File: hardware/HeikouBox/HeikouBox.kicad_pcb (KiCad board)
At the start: 2 copper layers, 100 x 100 mm, 193 parts, among them J101 5V, J201 Conn_02x05_Odd_Even, J202 Conn_02x08_Odd_Even, J301 DB15_Female_HighDensity_Mount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, J302 AudioJack3_SwitchTR, J501 Micro_SD_Card_TFP09-2-12B, J503 PS/2, Q301 MMBT3904, Q302 MMBT3904, Q303 MMBT3904, Q304 MMBT3904, Q305 MMBT3904, Q306 MMBT3904, Q307 MMBT3904, Q502 BSS138, Q503 BSS138, SW501 Left, SW502 Right, SW503 Up, SW504 Down, U101 LD1117S33TR, U102 LD1117S25TR, U103 LD1117S12TR, U201 HeikouBox-Core, U202 74HCU04, U401 K4S281632-UC60, U501 STM32-BluePill-Socket, Y201 14.31818MHz, Y202 28.37516MHz

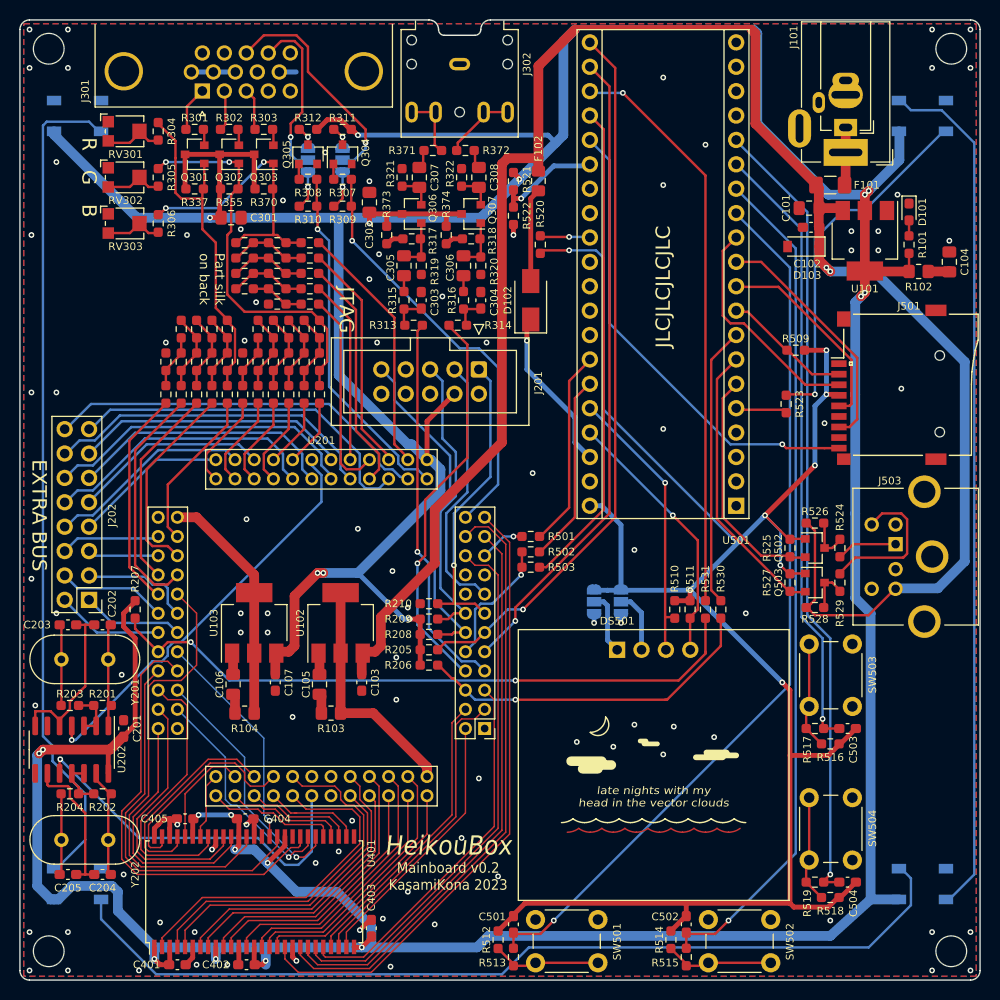
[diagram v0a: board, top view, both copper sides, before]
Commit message: Upload latest files
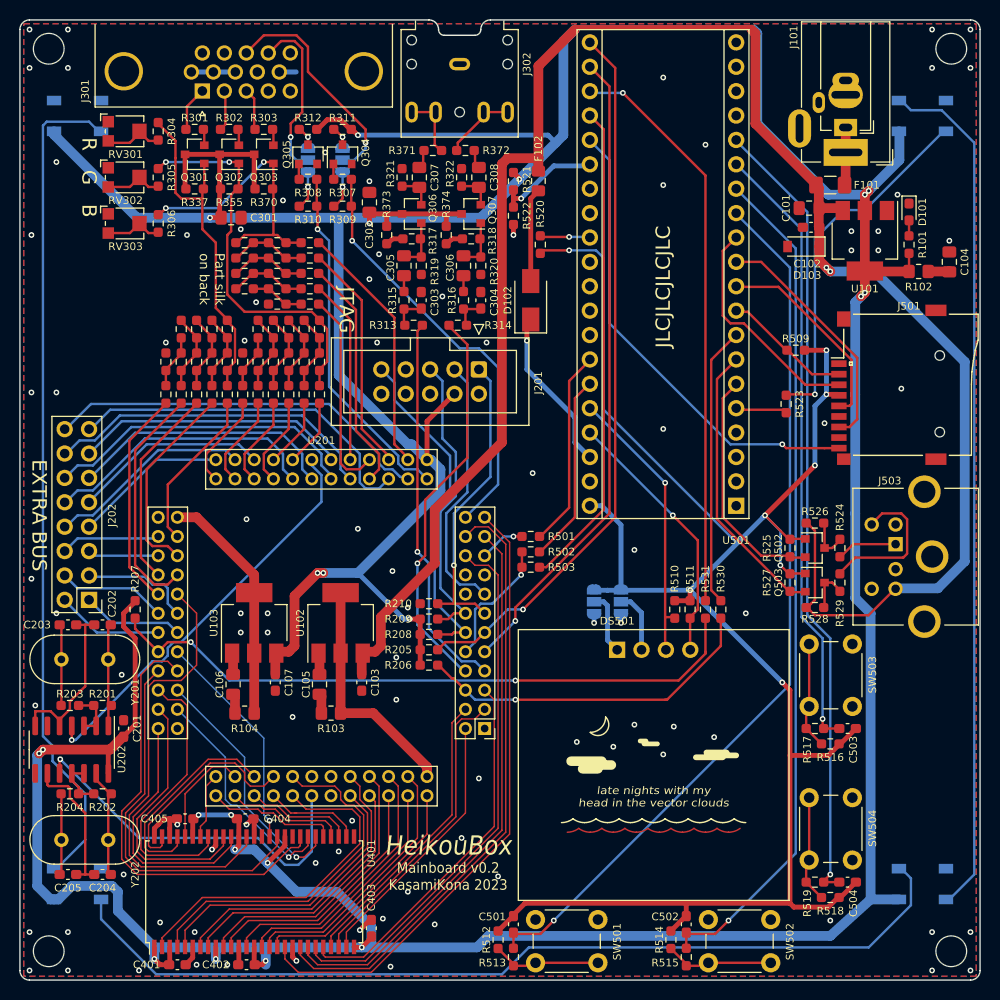
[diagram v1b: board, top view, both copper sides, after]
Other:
- net class Default removed
- net class Power removed
- net class Signal removed
